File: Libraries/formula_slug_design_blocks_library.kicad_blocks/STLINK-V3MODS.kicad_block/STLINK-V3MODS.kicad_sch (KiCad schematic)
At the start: 1 part

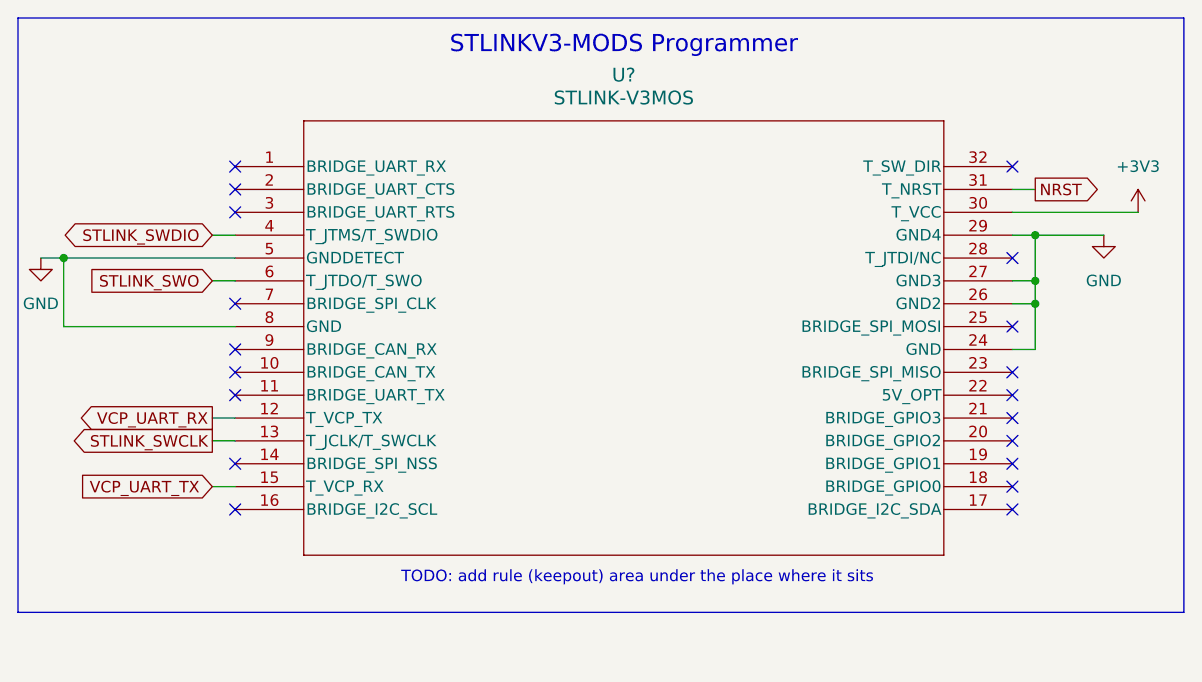
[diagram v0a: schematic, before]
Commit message: use snapeda cad files for stlinkv3-mods
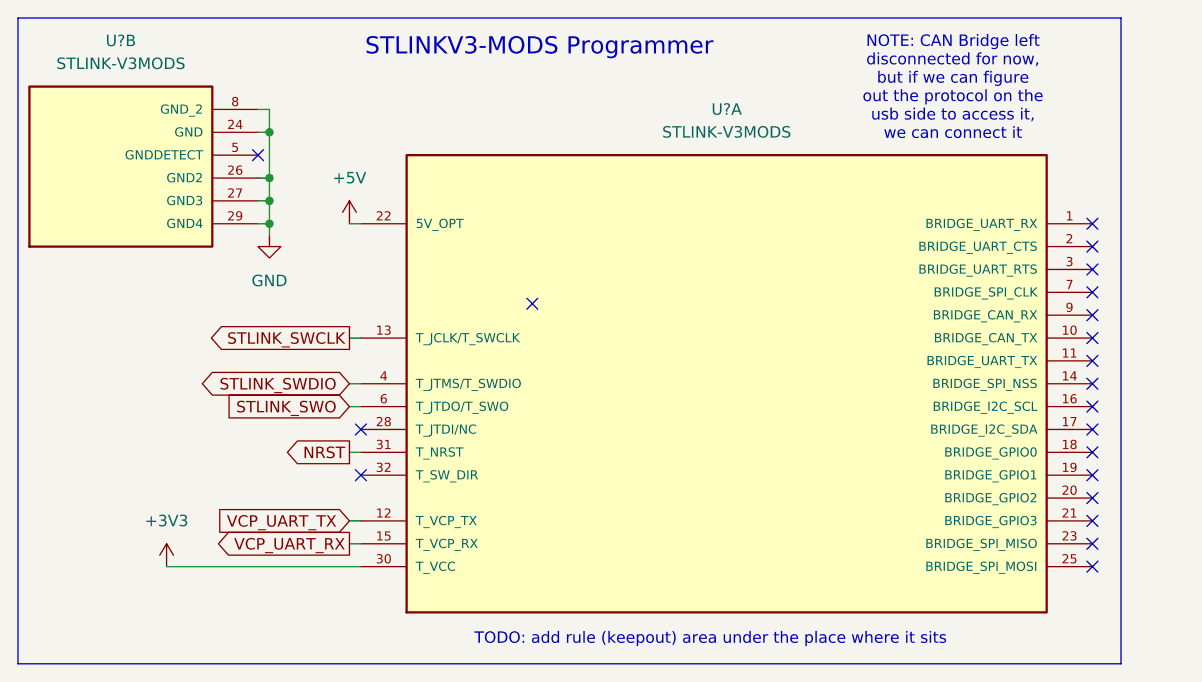
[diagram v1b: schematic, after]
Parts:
- removed U?: STLINK-V3MOS, mod_stlink-v3m_mb1467, symbol FS_4_Global_Symbol_Library:STLINK-V3MOS
- added U? (x2): STLINK-V3MODS, STLINK-V3MODS:MODULE_STLINK-V3MODS, symbol FS_4_Global_Symbol_Library:STLINK-V3MODS
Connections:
- net +3V3: now also U?.30 (T_VCC)
- net GND: now also U?.24 (GND), U?.26 (GND2), U?.27 (GND3), U?.29 (GND4), U?.8 (GND_2)
- net NRST: now also U?.31 (T_NRST)
- net STLINK_SWCLK: now also U?.13 (T_JCLK/T_SWCLK)
- net STLINK_SWDIO: now also U?.4 (T_JTMS/T_SWDIO)
- net STLINK_SWO: now also U?.6 (T_JTDO/T_SWO)
- net VCP_UART_RX: now also U?.15 (T_VCP_RX)
- net VCP_UART_TX: now also U?.12 (T_VCP_TX)
- new net +5V: U?.22 (5V_OPT)
- no-connect marks 19 -> 20
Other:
- note added: "NOTE: CAN Bridge left disconnected for now, but if we can figure out the protocol on the usb side to access it, we can connect it"

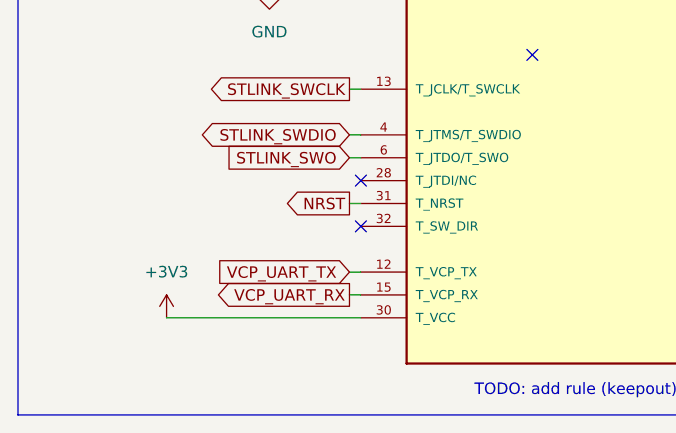
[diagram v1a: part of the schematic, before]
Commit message: fix rx and tx on stlinkv3-mods
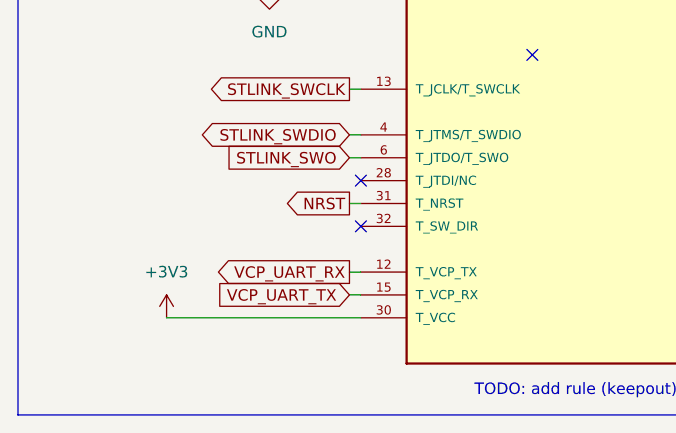
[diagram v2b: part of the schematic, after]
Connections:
- net VCP_UART_RX: now also U?.12 (T_VCP_TX); no longer U?.15 (T_VCP_RX)
- net VCP_UART_TX: now also U?.15 (T_VCP_RX); no longer U?.12 (T_VCP_TX)
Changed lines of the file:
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@@
+	(wire
+		(pts
+			(xy 74.93 80.01) (xy 76.2 80.01)
+		)
+		(stroke
+			(width 0)
+			(type default)
+		)
+	)
+	(wire
+		(pts
+			(xy 74.93 82.55) (xy 76.2 82.55)
+		)
+		(stroke
+			(width 0)
+			(type default)
+		)
+	)
 	(wire
 		(pts
@@
 	(wire
 		(pts
-			(xy 74.93 80.01) (xy 76.2 80.01)
-		)
-		(stroke
-			(width 0)
-			(type default)
-		)
-	)
-	(wire
-		(pts
 			(xy 74.93 72.39) (xy 76.2 72.39)
 		)
@@
 		(pts
 			(xy 64.77 36.83) (xy 66.04 36.83)
-		)
-		(stroke
-			(width 0)
-			(type default)
-		)
-	)
-	(wire
-		(pts
-			(xy 74.93 82.55) (xy 76.2 82.55)
 		)
 		(stroke
@@
 	(global_label "VCP_UART_RX"
 		(shape output)
-		(at 74.93 82.55 180)
-		(fields_autoplaced yes)
-		(effects
-			(font
-				(size 1.27 1.27)
-			)
-			(justify right)
-		)
-		(property "Intersheetrefs" "${INTERSHEET_REFS}"
-			(at 59.2448 82.55 0)
+		(at 74.93 80.01 180)
+		(fields_autoplaced yes)
+		(effects
+			(font
+				(size 1.27 1.27)
+			)
+			(justify right)
+		)
+		(property "Intersheetrefs" "${INTERSHEET_REFS}"
+			(at 59.2448 80.01 0)
 			(effects
 				(font
@@
 	(global_label "VCP_UART_TX"
 		(shape input)
-		(at 74.93 80.01 180)
-		(fields_autoplaced yes)
-		(effects
-			(font
-				(size 1.27 1.27)
-			)
-			(justify right)
-		)
-		(property "Intersheetrefs" "${INTERSHEET_REFS}"
-			(at 59.5472 80.01 0)
-			(effects
-				(font
+		(at 74.93 82.55 180)
+		(fields_autoplaced yes)
+		(effects
+			(font
+				(size 1.27 1.27)
+			)
+			(justify right)
+		)
+		(property "Intersheetrefs" "${INTERSHEET_REFS}"
+			(at 59.5472 82.55 0)
+			(effects
+				(font
